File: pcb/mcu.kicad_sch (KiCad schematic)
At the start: 29 parts, among them J1 RC555, J2 pa1010d, J4 USB_C_Receptacle_USB2.0_16P, J5 UART, Q1 AO3401A, SW2 BOOT, SW3 EN, U3 ESP32-S3-WROOM-1

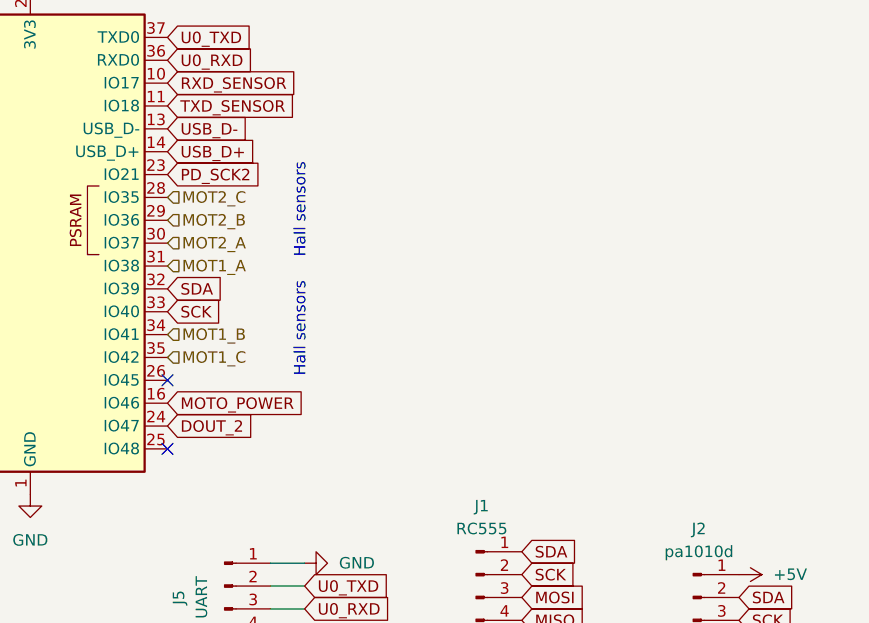
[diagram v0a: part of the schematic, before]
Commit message: update
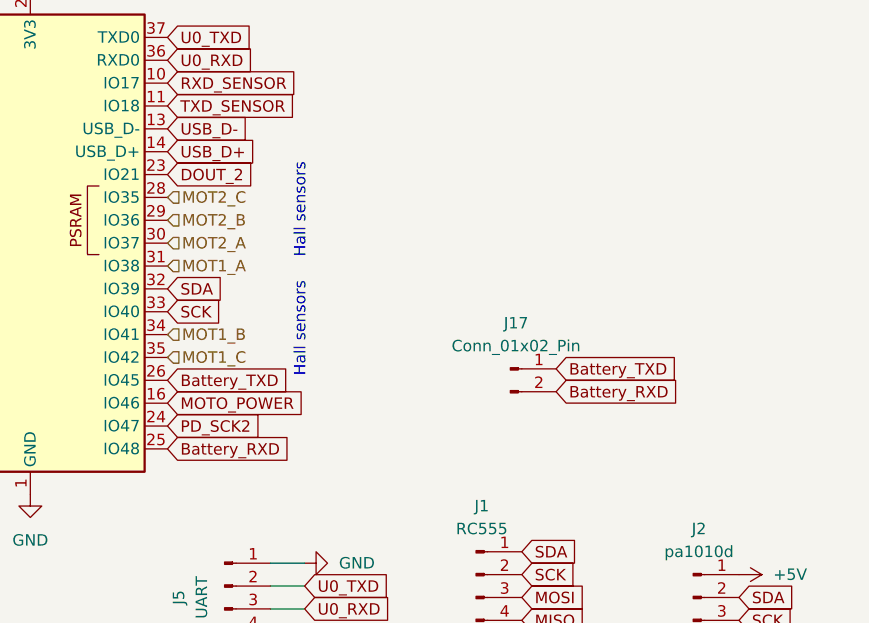
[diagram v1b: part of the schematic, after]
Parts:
- added J17: Conn_01x02_Pin, Connector_PinSocket_2.54mm:PinSocket_1x02_P2.54mm_Vertical, symbol Connector:Conn_01x02_Pin
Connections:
- net DOUT_2: now also U3.23 (IO21); no longer U3.24 (IO47)
- net PD_SCK2: now also U3.24 (IO47); no longer U3.23 (IO21)
- net Battery_RXD: now reaches U3.25 (IO48)
- net Battery_RXD: now also J17.2 (Pin_2)
- net Battery_TXD: now reaches U3.26 (IO45)
- net Battery_TXD: now also J17.1 (Pin_1)
- no-connect marks 5 -> 3
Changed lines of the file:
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@@
 		(at 72.39 67.31)
 	)
-	(no_connect
-		(at 78.74 148.59)
-	)
-	(no_connect
-		(at 78.74 156.21)
-	)
 	(wire
 		(pts
@@
 		)
 	)
+	(global_label "PD_SCK2"
+		(shape input)
+		(at 78.74 153.67 0)
+		(fields_autoplaced yes)
+		(effects
+			(font
+				(size 1.27 1.27)
+			)
+			(justify left)
+		)
+		(property "Intersheetrefs" "${INTERSHEET_REFS}"
+			(at 90.1918 153.67 0)
+			(hide yes)
+			(effects
+				(font
+					(size 1.27 1.27)
+				)
+				(justify left)
+			)
+		)
+	)
 	(global_label "EN"
 		(shape input)
@@
 		)
 	)
+	(global_label "Battery_TXD"
+		(shape input)
+		(at 121.92 147.32 0)
+		(fields_autoplaced yes)
+		(effects
+			(font
+				(size 1.27 1.27)
+			)
+			(justify left)
+		)
+		(property "Intersheetrefs" "${INTERSHEET_REFS}"
+			(at 136.0327 147.32 0)
+			(hide yes)
+			(effects
+				(font
+					(size 1.27 1.27)
+				)
+				(justify left)
+			)
+		)
+	)
+	(global_label "DOUT_2"
+		(shape input)
+		(at 78.74 125.73 0)
+		(fields_autoplaced yes)
+		(effects
+			(font
+				(size 1.27 1.27)
+			)
+			(justify left)
+		)
+		(property "Intersheetrefs" "${INTERSHEET_REFS}"
+			(at 88.8009 125.73 0)
+			(hide yes)
+			(effects
+				(font
+					(size 1.27 1.27)
+				)
+				(justify left)
+			)
+		)
+	)
 	(global_label "TXD_SENSOR"
 		(shape input)
@@
 		)
 	)
-	(global_label "DOUT_2"
-		(shape input)
-		(at 78.74 153.67 0)
-		(fields_autoplaced yes)
-		(effects
-			(font
-				(size 1.27 1.27)
-			)
-			(justify left)
-		)
-		(property "Intersheetrefs" "${INTERSHEET_REFS}"
-			(at 88.8009 153.67 0)
-			(hide yes)
-			(effects
-				(font
-					(size 1.27 1.27)
-				)
-				(justify left)
-			)
-		)
-	)
 	(global_label "SDA"
 		(shape input)
@@
 		)
 	)
-	(global_label "PD_SCK2"
-		(shape input)
-		(at 78.74 125.73 0)
-		(fields_autoplaced yes)
-		(effects
-			(font
-				(size 1.27 1.27)
-			)
-			(justify left)
-		)
-		(property "Intersheetrefs" "${INTERSHEET_REFS}"
-			(at 90.1918 125.73 0)
-			(hide yes)
-			(effects
-				(font
-					(size 1.27 1.27)
-				)
-				(justify left)
-			)
-		)
-	)
 	(global_label "U0_RXD"
 		(shape input)
@@
 		)
 	)
+	(global_label "Battery_RXD"
+		(shape input)
+		(at 121.92 149.86 0)
+		(fields_autoplaced yes)
+		(effects
+			(font
+				(size 1.27 1.27)
+			)
+			(justify left)
+		)
+		(property "Intersheetrefs" "${INTERSHEET_REFS}"
+			(at 136.3351 149.86 0)
+			(hide yes)
+			(effects
+				(font
+					(size 1.27 1.27)
+				)
+				(justify left)
+			)
+		)
+	)
 	(global_label "USB_D-"
 		(shape input)
@@
 					(size 1.27 1.27)
 				)
+			)
+		)
+	)
+	(global_label "Battery_TXD"
+		(shape input)
+		(at 78.74 148.59 0)
+		(fields_autoplaced yes)
+		(effects
+			(font
+				(size 1.27 1.27)
+			)
+			(justify left)
+		)
+		(property "Intersheetrefs" "${INTERSHEET_REFS}"
+			(at 92.8527 148.59 0)
+			(hide yes)
+			(effects
+				(font
+					(size 1.27 1.27)
+				)
+				(justify left)
 			)
 		)
@@
 				)
 				(justify right)
+			)
+		)
+	)
+	(global_label "Battery_RXD"
+		(shape input)
+		(at 78.74 156.21 0)
+		(fields_autoplaced yes)
+		(effects
+			(font
+				(size 1.27 1.27)
+			)
+			(justify left)
+		)
+		(property "Intersheetrefs" "${INTERSHEET_REFS}"
+			(at 93.1551 156.21 0)
+			(hide yes)
+			(effects
+				(font
+					(size 1.27 1.27)
+				)
+				(justify left)
 			)
 		)
@@
 					(unit 1)
 				)
+			)
+		)
+	)
+	(symbol
+		(lib_id "Connector:Conn_01x02_Pin")
+		(at 116.84 147.32 0)
+		(unit 1)
+		(exclude_from_sim no)
+		(in_bom yes)
+		(on_board yes)
+		(dnp no)
+		(fields_autoplaced yes)
+		(property "Reference" "J17"
+			(at 117.475 142.24 0)
+			(effects
+				(font
+					(size 1.27 1.27)
+				)
+			)
+		)
+		(property "Value" "Conn_01x02_Pin"
+			(at 117.475 144.78 0)
+			(effects
+				(font
+					(size 1.27 1.27)
+				)
+			)
+		)
+		(property "Footprint" "Connector_PinSocket_2.54mm:PinSocket_1x02_P2.54mm_Vertical"
+			(at 116.84 147.32 0)
+			(hide yes)
+			(effects
+				(font
+					(size 1.27 1.27)
+				)
+			)
+		)
+		(property "Datasheet" ""
+			(at 116.84 147.32 0)
+			(hide yes)
+			(effects
+				(font
+					(size 1.27 1.27)
+				)
+			)
+		)
+		(property "Description" "Generic connector, single row, 01x02, script generated"
+			(at 116.84 147.32 0)
+			(hide yes)
+			(effects
+				(font
+					(size 1.27 1.27)
+				)
+			)
+		)
+		(pin "2"
+		)
+		(pin "1"
+		)
+		(instances
+			(project ""
+				(path "/5cdb5c16-5e05-458b-86f0-906cf8114d7e/5f743cab-9820-4aca-8ca5-f45b69affbe2"
+					(reference "J17")
+					(unit 1)
+				)
